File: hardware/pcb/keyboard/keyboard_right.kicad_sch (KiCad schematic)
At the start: 29 parts, among them J1 SM04B-SRSS-TB, J2 PJ320D, J3 HRO_TYPE-C-31-M-12, J4 FFC Connector, SW29 PTS845, U3 DT1446-04S, U4 XC6220B331MR-G, U5 STM32G431KBTx, Y1 8MHz

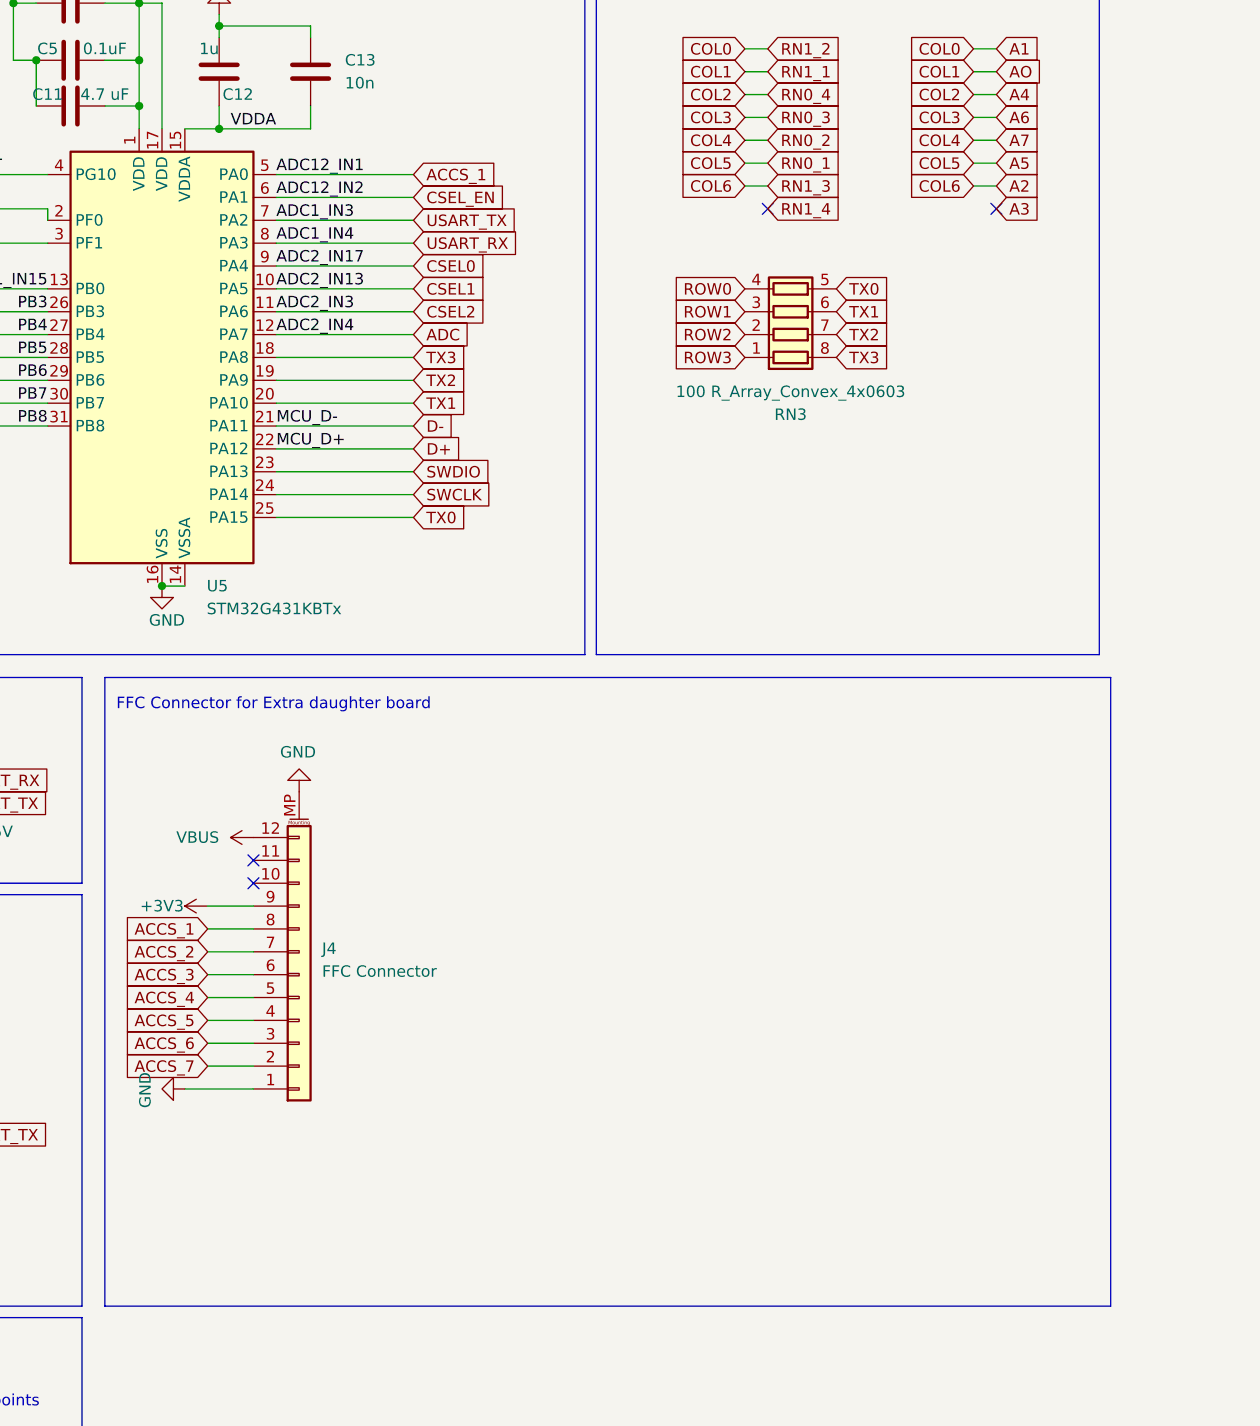
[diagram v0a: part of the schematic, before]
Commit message: usb hib init
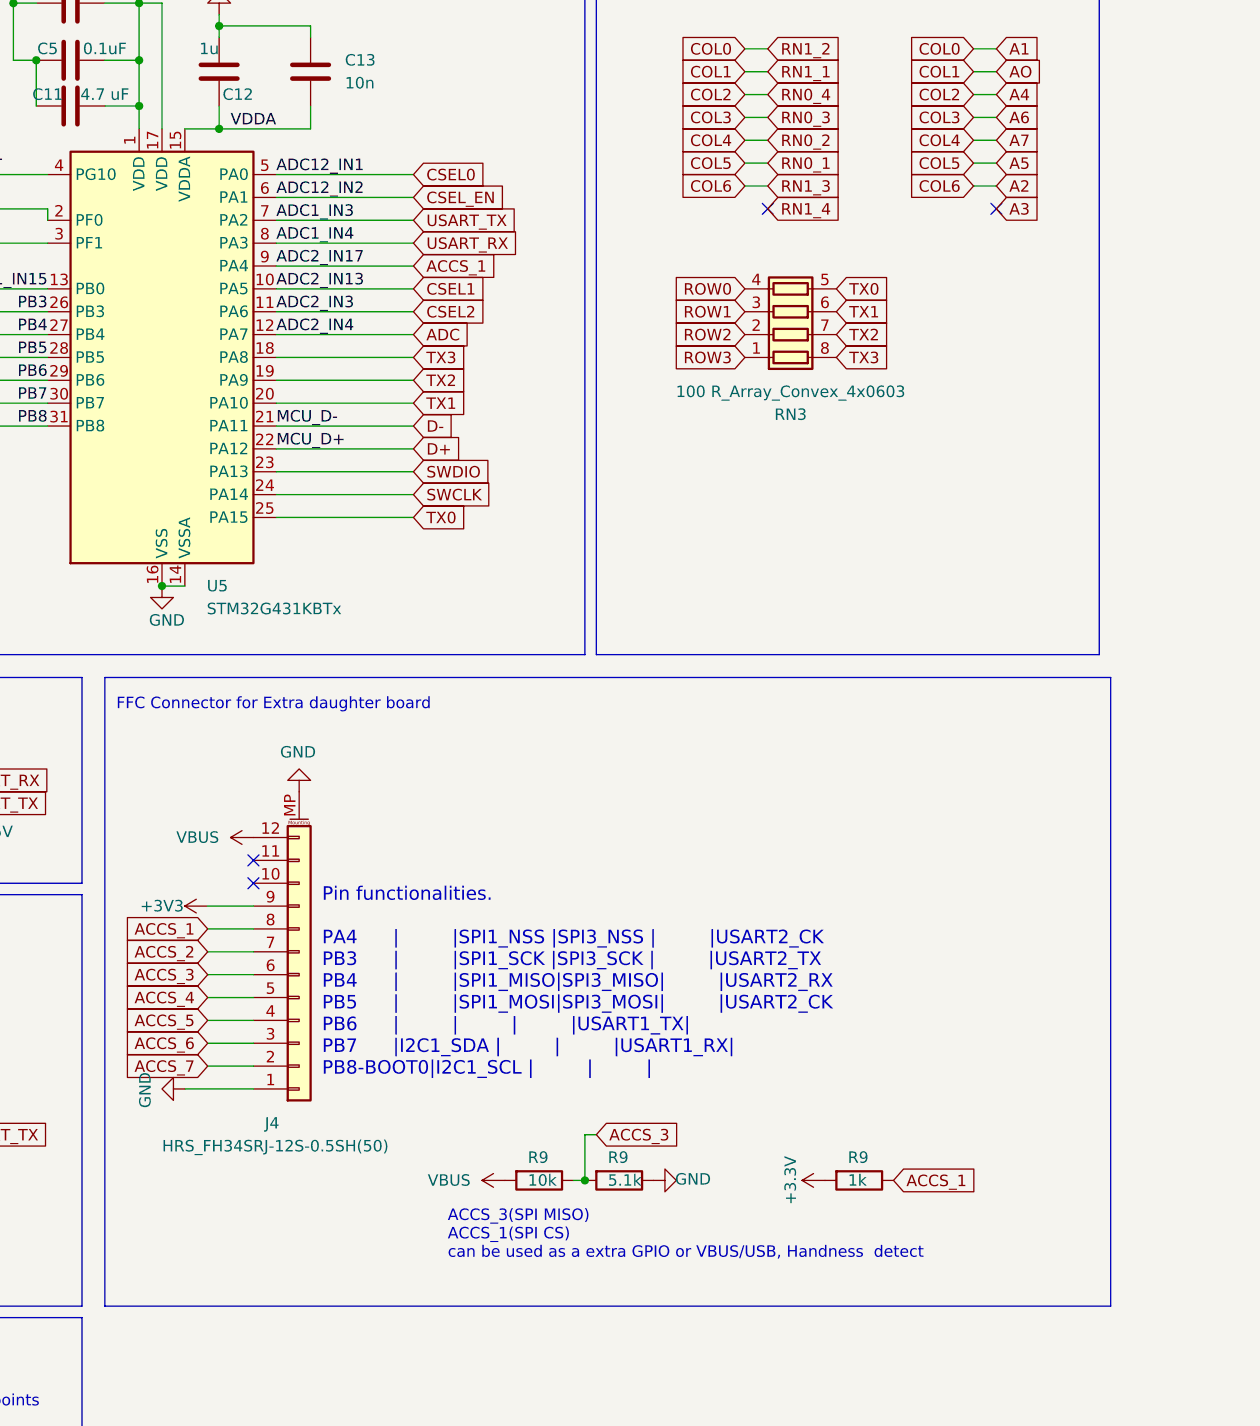
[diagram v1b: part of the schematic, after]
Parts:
- added R9: 1k, PCM_Resistor_SMD_AKL:R_0603_1608Metric, symbol Device:R
- added R9: 10k, PCM_Resistor_SMD_AKL:R_0603_1608Metric, symbol Device:R
- added R9: 5.1k, PCM_Resistor_SMD_AKL:R_0603_1608Metric, symbol Device:R
- J4: value FFC Connector -> HRS_FH34SRJ-12S-0.5SH(50)
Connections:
- net +3V3: now also R9.2
- net ACCS_1: now also U5.9 (PA4), R9.1; no longer U5.5 (PA0)
- net ACCS_3: now also R9.1, R9.2
- net CSEL0: now also U5.5 (PA0); no longer U5.9 (PA4)
- net GND: now also R9.1
- net VBUS: now also R9.2
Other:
- note added: "ACCS_3(SPI MISO) ACCS_1(SPI CS) can be used as a extra GPIO or VBUS/USB, Handness detect"
- note added: "Pin functionalities. PA4 | |SPI1_NSS |SPI3_NSS | |USART2_CK PB3 | |SPI1_SCK |SPI3_SCK | |USART2_TX PB4 | |SPI1_MISO|SPI3_MISO| |USART2_RX PB5 | |SPI1_MOSI|SPI3_MOSI| |USART2_CK PB6 | | | |USART1_TX| PB7 |I2C1_SDA | | |USART1_RX| PB8-BOOT0|I2C1_SCL | | |"

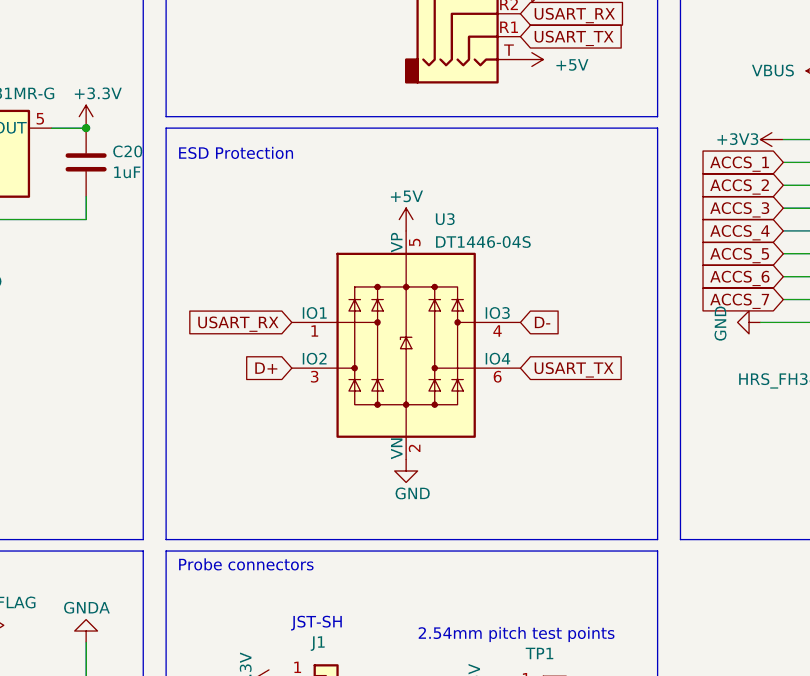
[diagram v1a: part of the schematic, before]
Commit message: preproduction
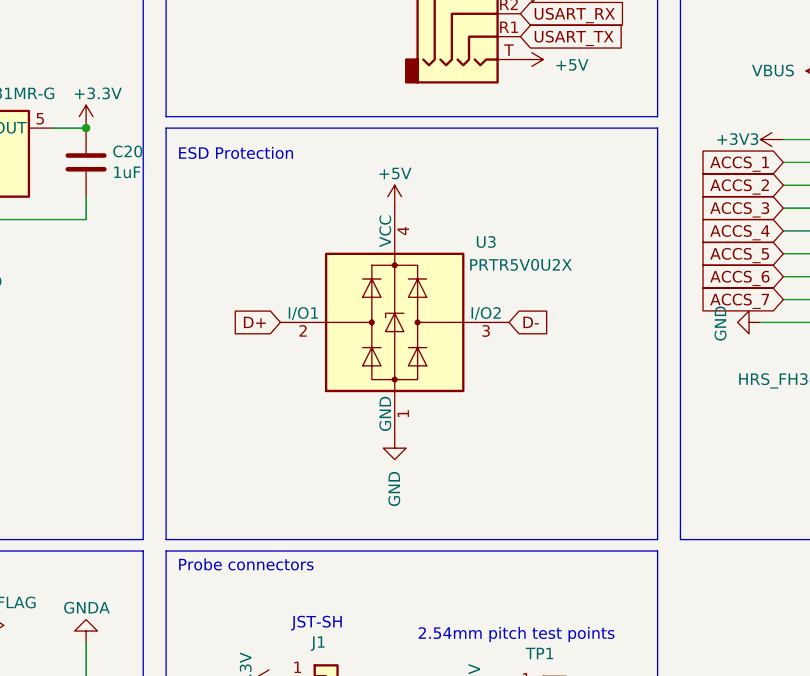
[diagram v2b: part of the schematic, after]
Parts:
- removed U3: DT1446-04S, PCM_Package_TO_SOT_SMD_AKL:SOT-363_SC-70-6_Handsoldering, symbol Power_Protection:SRV05-4
- added U3: PRTR5V0U2X, PCM_Package_TO_SOT_SMD_AKL:SOT-143, symbol Power_Protection:PRTR5V0U2X
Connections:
- net +5V: now also U3.4 (VCC)
- net D+: now also U3.2 (I/O1)
- net D-: now also U3.3 (I/O2)
- net GND: now also U3.1 (GND)
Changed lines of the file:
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@@
-    )
-  )
-  (global_label "D-" (shape input) (at 154.94 139.7 0) (fields_autoplaced)
-    (effects (font (size 1.27 1.27)) (justify left))
-    (property "Intersheetrefs" "${INTERSHEET_REFS}" (at 159.1876 139.7 0)
-      (effects (font (size 1.27 1.27)) (justify left) hide)
     )
   )
@@
     )
   )
-  (global_label "USART_TX" (shape input) (at 154.94 144.78 0) (fields_autoplaced)
+  (global_label "D-" (shape input) (at 153.67 139.7 0) (fields_autoplaced)
     (effects (font (size 1.27 1.27)) (justify left))
-    (property "Intersheetrefs" "${INTERSHEET_REFS}" (at 165.6048 144.78 0)
+    (property "Intersheetrefs" "${INTERSHEET_REFS}" (at 157.9176 139.7 0)
       (effects (font (size 1.27 1.27)) (justify left) hide)
     )
@@
     (property "Intersheetrefs" "${INTERSHEET_REFS}" (at 253.8362 24.13 0)
       (effects (font (size 1.27 1.27)) (justify left) hide)
+    )
+  )
+  (global_label "D+" (shape input) (at 128.27 139.7 180) (fields_autoplaced)
+    (effects (font (size 1.27 1.27)) (justify right))
+    (property "Intersheetrefs" "${INTERSHEET_REFS}" (at 124.0224 139.7 0)
+      (effects (font (size 1.27 1.27)) (justify right) hide)
     )
   )
@@
     )
   )
-  (global_label "USART_RX" (shape input) (at 129.54 139.7 180) (fields_autoplaced)
-    (effects (font (size 1.27 1.27)) (justify right))
-    (property "Intersheetrefs" "${INTERSHEET_REFS}" (at 118.8752 139.7 0)
-      (effects (font (size 1.27 1.27)) (justify right) hide)
-    )
-  )
   (global_label "TX2" (shape input) (at 254 55.88 0) (fields_autoplaced)
     (effects (font (size 1.27 1.27)) (justify left))
@@
     (effects (font (size 1.27 1.27)) (justify right))
     (property "Intersheetrefs" "${INTERSHEET_REFS}" (at 237.4533 53.34 0)
-      (effects (font (size 1.27 1.27)) (justify right) hide)
-    )
-  )
-  (global_label "D+" (shape input) (at 129.54 144.78 180) (fields_autoplaced)
-    (effects (font (size 1.27 1.27)) (justify right))
-    (property "Intersheetrefs" "${INTERSHEET_REFS}" (at 125.2924 144.78 0)
       (effects (font (size 1.27 1.27)) (justify right) hide)
     )
@@
     )
   )
-  (symbol (lib_id "power:GND") (at 142.24 154.94 0) (mirror y) (unit 1)
-    (in_bom yes) (on_board yes) (dnp no)
-    (property "Reference" "#PWR022" (at 142.24 161.29 0)
-      (effects (font (size 1.27 1.27)) hide)
-    )
-    (property "Value" "GND" (at 140.97 158.75 0)
-      (effects (font (size 1.27 1.27)) (justify right))
-    )
-    (property "Footprint" "" (at 142.24 154.94 0)
-      (effects (font (size 1.27 1.27)) hide)
-    )
-    (property "Datasheet" "" (at 142.24 154.94 0)
-      (effects (font (size 1.27 1.27)) hide)
-    )
-    (pin "1")
-    (instances
-      (project "keyboard_right"
-        (path "/852dabbf-de45-4470-8176-59d37a754407"
-          (reference "#PWR022") (unit 1)
-        )
-      )
-      (project "EC60-Rev_1_1"
-        (path "/e63e39d7-6ac0-4ffd-8aa3-1841a4541b55"
-          (reference "#PWR020") (unit 1)
-        )
-      )
-    )
-  )
   (symbol (lib_id "PCM_Diode_Schottky_AKL:1N5818") (at 68.58 118.11 0) (unit 1)
     (in_bom yes) (on_board yes) (dnp no)
@@
     )
   )
+  (symbol (lib_id "Power_Protection:PRTR5V0U2X") (at 140.97 139.7 0) (unit 1)
+    (in_bom yes) (on_board yes) (dnp no)
+    (property "Reference" "U3" (at 151.13 130.81 0)
+      (effects (font (size 1.27 1.27)))
+    )
+    (property "Value" "PRTR5V0U2X" (at 154.94 133.35 0)
+      (effects (font (size 1.27 1.27)))
+    )
+    (property "Footprint" "PCM_Package_TO_SOT_SMD_AKL:SOT-143" (at 142.494 139.7 0)
+      (effects (font (size 1.27 1.27)) hide)
+    )
+    (property "Datasheet" "https://assets.nexperia.com/documents/data-sheet/PRTR5V0U2X.pdf" (at 142.494 139.7 0)
+      (effects (font (size 1.27 1.27)) hide)
+    )
+    (property "LCSC" "C2827688" (at 140.97 139.7 0)
+      (effects (font (size 1.27 1.27)) hide)
+    )
+    (pin "1")
+    (pin "2")
+    (pin "3")
+    (pin "4")
+    (instances
+      (project "keyboard_right"
+        (path "/852dabbf-de45-4470-8176-59d37a754407"
+          (reference "U3") (unit 1)
+        )
+      )
+      (project "EC60-Rev_1_1"
+        (path "/e63e39d7-6ac0-4ffd-8aa3-1841a4541b55"
+          (reference "D1") (unit 1)
+        )
+      )
+    )
+  )
   (symbol (lib_id "Device:C") (at 185.42 26.67 180) (unit 1)
     (in_bom yes) (on_board yes) (dnp no)
@@
     )
   )
+  (symbol (lib_id "power:GND") (at 140.97 152.4 0) (mirror y) (unit 1)
+    (in_bom yes) (on_board yes) (dnp no)
+    (property "Reference" "#PWR022" (at 140.97 158.75 0)
+      (effects (font (size 1.27 1.27)) hide)
+    )
+    (property "Value" "GND" (at 140.97 156.21 90)
+      (effects (font (size 1.27 1.27)) (justify right))
+    )
+    (property "Footprint" "" (at 140.97 152.4 0)
+      (effects (font (size 1.27 1.27)) hide)
+    )
+    (property "Datasheet" "" (at 140.97 152.4 0)
+      (effects (font (size 1.27 1.27)) hide)
+    )
+    (pin "1")
+    (instances
+      (project "keyboard_right"
+        (path "/852dabbf-de45-4470-8176-59d37a754407"
+          (reference "#PWR022") (unit 1)
+        )
+      )
+      (project "EC60-Rev_1_1"
+        (path "/e63e39d7-6ac0-4ffd-8aa3-1841a4541b55"
+          (reference "#PWR020") (unit 1)
+        )
+      )
+    )
+  )
   (symbol (lib_id "Device:C") (at 127 49.53 90) (mirror x) (unit 1)
     (in_bom yes) (on_board yes) (dnp no)
@@
         (path "/e63e39d7-6ac0-4ffd-8aa3-1841a4541b55"
           (reference "#PWR022") (unit 1)
-        )
-      )
-    )
-  )
-  (symbol (lib_id "power:+5V") (at 142.24 129.54 0) (unit 1)
-    (in_bom yes) (on_board yes) (dnp no)
-    (property "Reference" "#PWR020" (at 142.24 133.35 0)
-      (effects (font (size 1.27 1.27)) hide)
-    )
-    (property "Value" "+5V" (at 142.24 125.73 0)
-      (effects (font (size 1.27 1.27)))
-    )
-    (property "Footprint" "" (at 142.24 129.54 0)
-      (effects (font (size 1.27 1.27)) hide)
-    )
-    (property "Datasheet" "" (at 142.24 129.54 0)
-      (effects (font (size 1.27 1.27)) hide)
-    )
-    (pin "1")
-    (instances
-      (project "keyboard_right"
-        (path "/852dabbf-de45-4470-8176-59d37a754407"
-          (reference "#PWR020") (unit 1)
-        )
-      )
-      (project "EC60"
-        (path "/e63e39d7-6ac0-4ffd-8aa3-1841a4541b55"
-          (reference "#PWR010") (unit 1)
         )
       )
@@
     )
   )
-  (symbol (lib_id "Power_Protection:SRV05-4") (at 142.24 142.24 0) (unit 1)
-    (in_bom yes) (on_board yes) (dnp no) (fields_autoplaced)
-    (property "Reference" "U3" (at 145.3897 128.27 0)
-      (effects (font (size 1.27 1.27)) (justify left))
-    )
-    (property "Value" "DT1446-04S" (at 145.3897 130.81 0)
-      (effects (font (size 1.27 1.27)) (justify left))
-    )
-    (property "Footprint" "PCM_Package_TO_SOT_SMD_AKL:SOT-363_SC-70-6_Handsoldering" (at 160.02 153.67 0)
-      (effects (font (size 1.27 1.27)) hide)
-    )
-    (property "Datasheet" "http://www.onsemi.com/pub/Collateral/SRV05-4-D.PDF" (at 142.24 142.24 0)
-      (effects (font (size 1.27 1.27)) hide)
-    )
-    (property "Comment" "" (at 142.24 142.24 0)
-      (effects (font (size 1.27 1.27)) hide)
-    )
-    (pin "1")
-    (pin "2")
-    (pin "3")
-    (pin "4")
-    (pin "5")
-    (pin "6")
-    (instances
-      (project "keyboard_right"
-        (path "/852dabbf-de45-4470-8176-59d37a754407"
-          (reference "U3") (unit 1)
-        )
-      )
+  (symbol (lib_id "power:+5V") (at 140.97 127 0) (unit 1)
+    (in_bom yes) (on_board yes) (dnp no)
+    (property "Reference" "#PWR020" (at 140.97 130.81 0)
+      (effects (font (size 1.27 1.27)) hide)
+    )
+    (property "Value" "+5V" (at 140.97 123.19 0)
+      (effects (font (size 1.27 1.27)))
+    )
+    (property "Footprint" "" (at 140.97 127 0)
+      (effects (font (size 1.27 1.27)) hide)
+    )
+    (property "Datasheet" "" (at 140.97 127 0)
+      (effects (font (size 1.27 1.27)) hide)
+    )
+    (pin "1")
+    (instances
+      (project "keyboard_right"
+        (path "/852dabbf-de45-4470-8176-59d37a754407"
+          (reference "#PWR020") (unit 1)
+        )
+      )
+      (project "EC60"
+        (path "/e63e39d7-6ac0-4ffd-8aa3-1841a4541b55"
+          (reference "#PWR010") (unit 1)
+        )
+      )
